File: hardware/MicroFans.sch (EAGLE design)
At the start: 29 parts, among them IC4 ATMEGA328P, IC7 OPA4251UA, J1 COMPUTER-PERIPHERAL-POWERVERT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, Y1 20Mhz

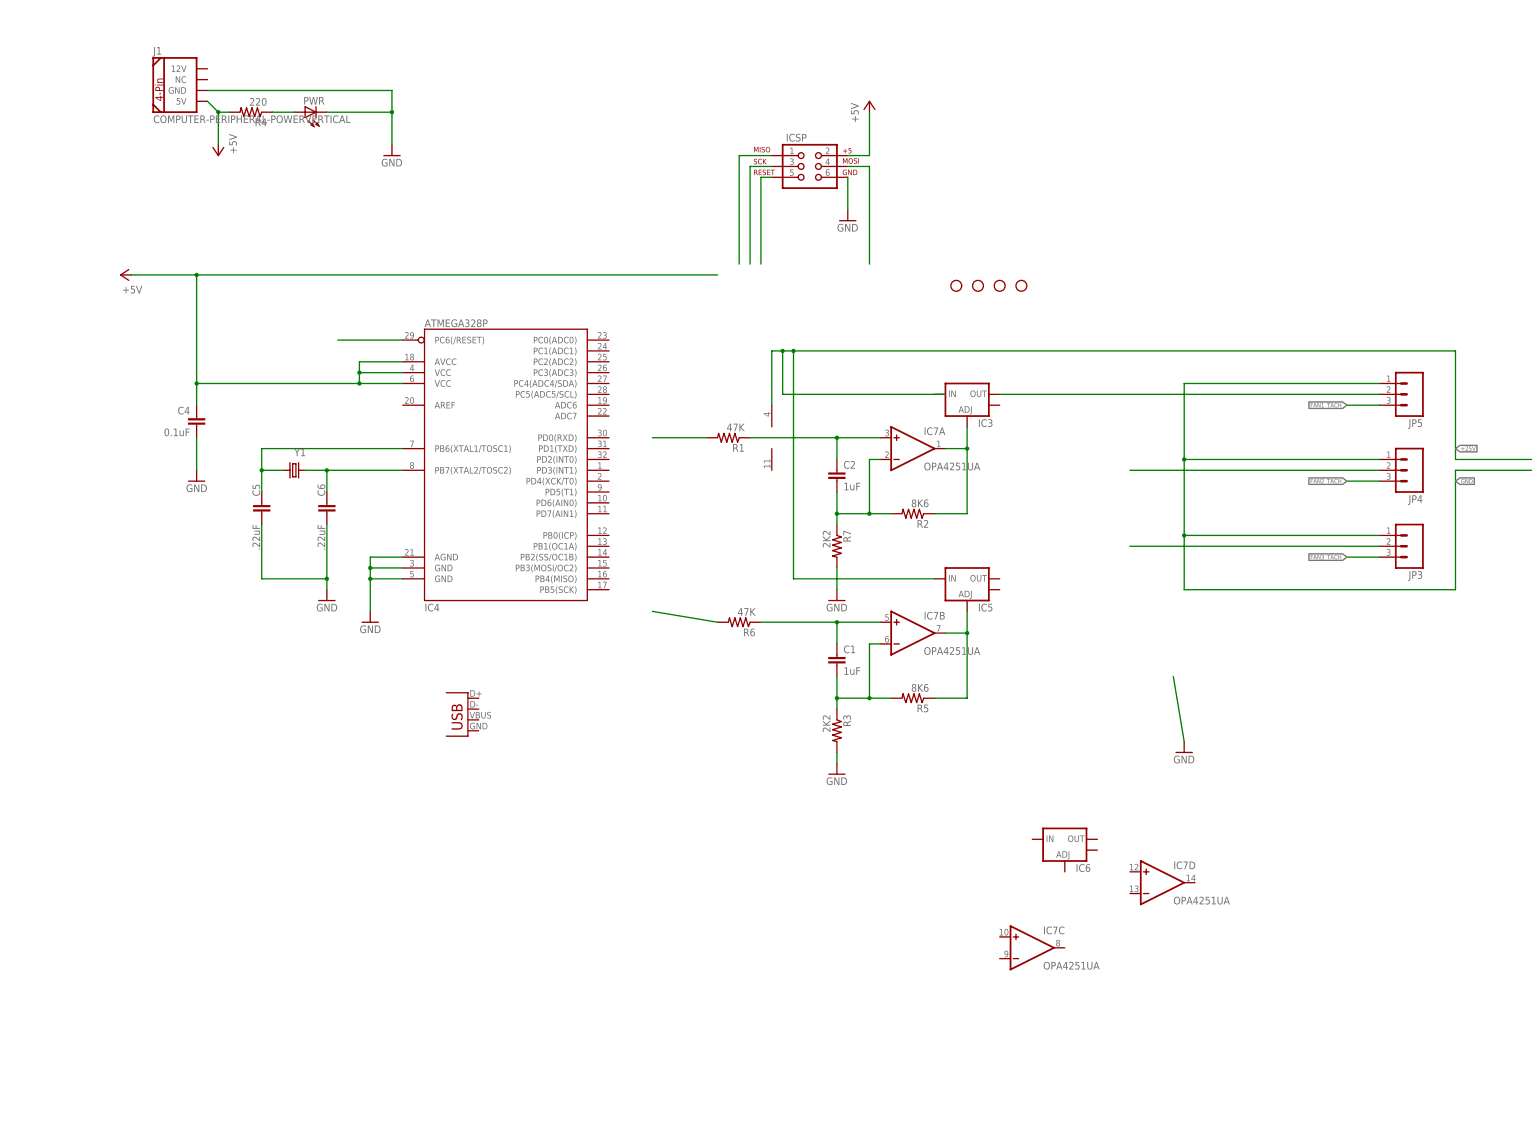
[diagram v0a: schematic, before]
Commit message: Update board
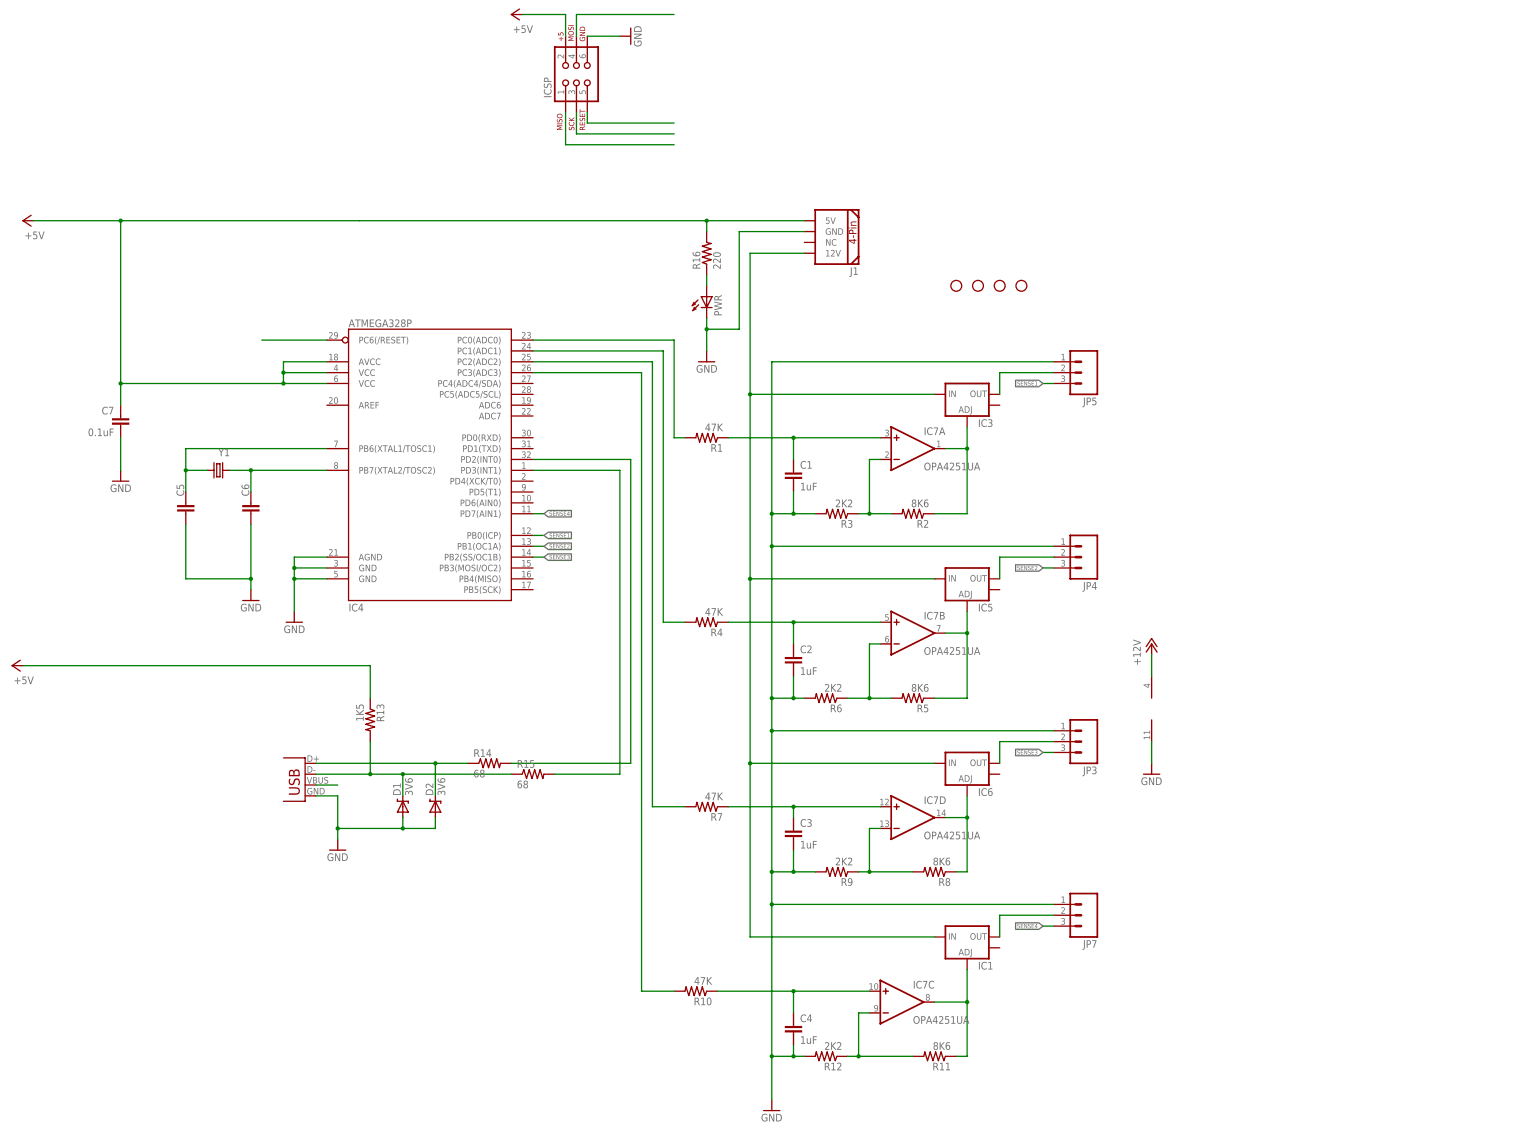
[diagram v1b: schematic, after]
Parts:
- added C3: 1uF, SparkFun-Capacitors:CAP0805
- added C7: 0.1uF, SparkFun-Passives:CAP1206
- added D1, D2: 3V6, SparkFun-DiscreteSemi:DIODE-ZENER-BZT52
- added IC1: (no value), SparkFun-PowerIC:V_REG_LM1117SOT223
- added JP7: (no value), SparkFun-Connectors:M03POLAR
- added R10: 47K, SparkFun-Passives:RESISTOR0805-RES
- added R11, R8: 8K6, SparkFun-Resistors:RESISTOR1206
- added R12, R9: 2K2, SparkFun-Resistors:RESISTOR1206
- added R13: 1K5, SparkFun-Passives:RESISTOR1206
- added R14, R15: 68, SparkFun-Passives:RESISTOR1206
- added R16: 220, SparkFun-Resistors:RESISTOR1206
- C1, C2: device SparkFun-Capacitors:CAPKIT -> SparkFun-Capacitors:CAP0805
- C4: value 0.1uF -> 1uF; device SparkFun-Capacitors:CAPKIT -> SparkFun-Capacitors:CAP0805
- C5, C6: device SparkFun-Capacitors:CAPKIT -> SparkFun-Passives:CAP1206
- JP1: value USB-A-S -> USB-A-SMD; device SparkFun-Connectors:USB-A-S -> SparkFun-Connectors:USB-A-SMD
- R1: device SparkFun-Resistors:RESISTOR1206 -> SparkFun-Passives:RESISTOR0805-RES
- R4: value 220 -> 47K; device SparkFun-Resistors:RESISTOR1206 -> SparkFun-Passives:RESISTOR0805-RES
- R6: value 47K -> 2K2
- R7: value 2K2 -> 47K; device SparkFun-Resistors:RESISTOR1206 -> SparkFun-Passives:RESISTOR0805-RES
- Y1: value 20Mhz -> 16MHZ
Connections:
- removed net +25V: IC5.IN
- removed net FAN1_TACH: JP5.3
- removed net FAN2_TACH: JP4.3
- removed net FAN3_TACH: JP3.3
- new net +12V: IC1.IN, IC3.IN, IC5.IN, IC6.IN, IC7P.V+, J1.12V
- new net N$1: IC1.OUT, JP7.2
- new net N$19: IC6.ADJ, IC7D.OUT, R8.1
- new net N$20: IC7D.-IN, R8.2, R9.1
- new net N$21: C3.1, IC7D.+IN, R7.1
- new net N$22: IC7C.-IN, R11.2, R12.1
- new net N$23: IC4.PC2(ADC2), R7.2
- new net N$24: C4.1, IC7C.+IN, R10.1
- new net N$25: IC1.ADJ, IC7C.OUT, R11.1
- new net N$26: D1.C, JP1.D-, R13.2, R15.1
- new net N$27: JP1.VBUS
- new net N$28: D2.C, JP1.D+, R14.1
- new net N$29: IC4.PD2(INT0), R14.2
- new net N$30: IC4.PD3(INT1), R15.2
- new net N$33: J1.5V, R16.2
- new net N$34: IC4.PC3(ADC3), R10.2
- new net SENSE1: IC4.PB0(ICP), JP5.3
- new net SENSE2: IC4.PB1(OC1A), JP4.3
- new net SENSE3: IC4.PB2(SS/OC1B), JP3.3
- new net SENSE4: IC4.PD7(AIN1), JP7.3
- net +5V: now also C7.1, R13.1; no longer C4.1, J1.5V, R4.2
- net GND: now also C1.2, C2.2, C3.2, C7.2, D1.A, D2.A, IC7P.V-, JP1.GND, JP7.1, R12.2, R6.2, R9.2; no longer R7.2
- net N$12: now also IC4.PC1(ADC1), R4.2; no longer R6.2
- net N$13: now also IC6.OUT, JP3.2; no longer JP4.2
- net N$15: now also C1.1; no longer C2.1
- net N$16: now also R3.1; no longer C2.2, R7.1
- net N$17: now also C2.1, R4.1; no longer C1.1, R6.1
- net N$18: now also R6.1; no longer C1.2, R3.1
- net N$5: now also IC4.PC0(ADC0)
- net N$7: now also R16.1; no longer R4.1
- net N$8: now also IC5.OUT, JP4.2; no longer JP3.2
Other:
- moved on the sheet: C1, C2, C4, C5, C6, IC4, IC6, IC7C, IC7D, ICSP, J1, JP3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
